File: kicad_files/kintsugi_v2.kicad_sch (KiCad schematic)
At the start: 164 parts, among them J1 Conn_01x04, J2 Conn_01x04, J3 AudioJack4, J4 AudioJack4, SW1 RotaryEncoder_Switch, SW2 SW_Push, U1 ProMicro, U2 MCP23017_SP

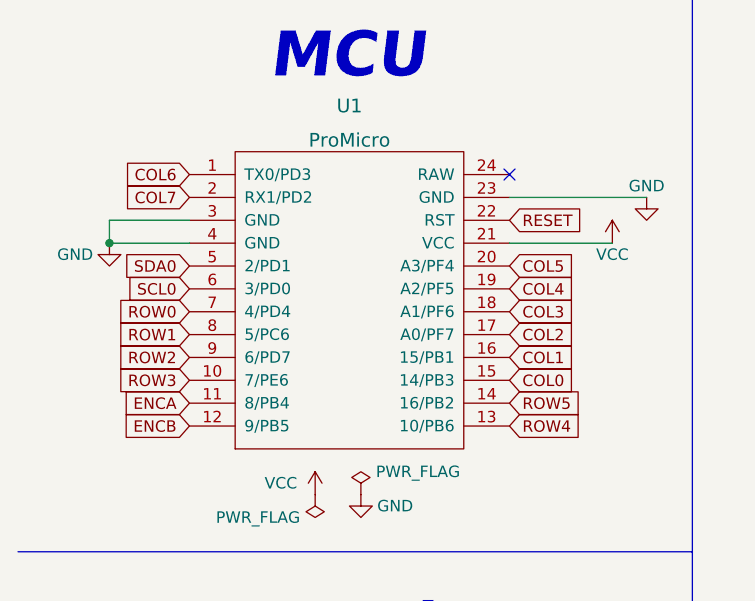
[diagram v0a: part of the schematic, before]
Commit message: Routed rows of the right side (down view) to the MCU.
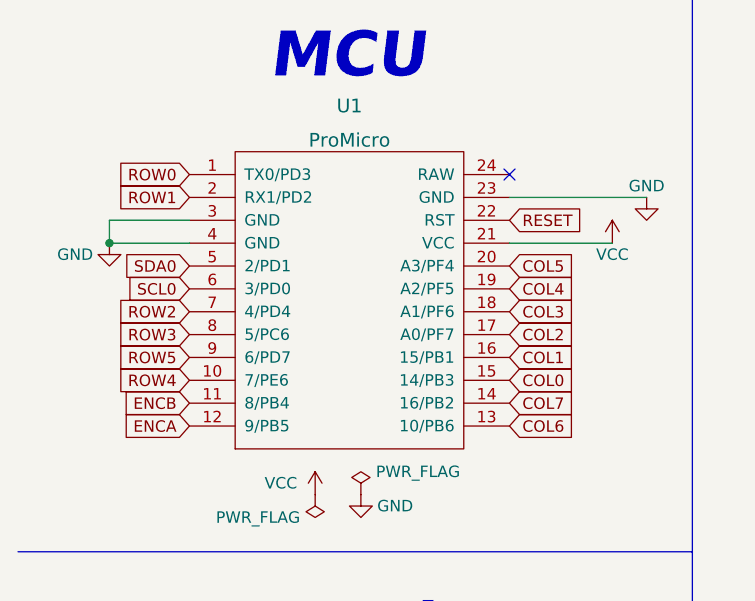
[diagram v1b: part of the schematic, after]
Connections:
- net COL6: now also U1.13 (10/PB6); no longer U1.1 (TX0/PD3)
- net COL7: now also U1.14 (16/PB2); no longer U1.2 (RX1/PD2)
- net ENCA: now also U1.12 (9/PB5); no longer U1.11 (8/PB4)
- net ENCB: now also U1.11 (8/PB4); no longer U1.12 (9/PB5)
- net ROW0: now also U1.1 (TX0/PD3); no longer U1.7 (4/PD4)
- net ROW1: now also U1.2 (RX1/PD2); no longer U1.8 (5/PC6)
- net ROW2: now also U1.7 (4/PD4); no longer U1.9 (6/PD7)
- net ROW3: now also U1.8 (5/PC6); no longer U1.10 (7/PE6)
- net ROW4: now also U1.10 (7/PE6); no longer U1.13 (10/PB6)
- net ROW5: now also U1.9 (6/PD7); no longer U1.14 (16/PB2)
